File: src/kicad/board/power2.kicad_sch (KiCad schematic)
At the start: 12 parts, among them Q1 DMG2301L, SW6 Enable BAT, U3 BQ25172

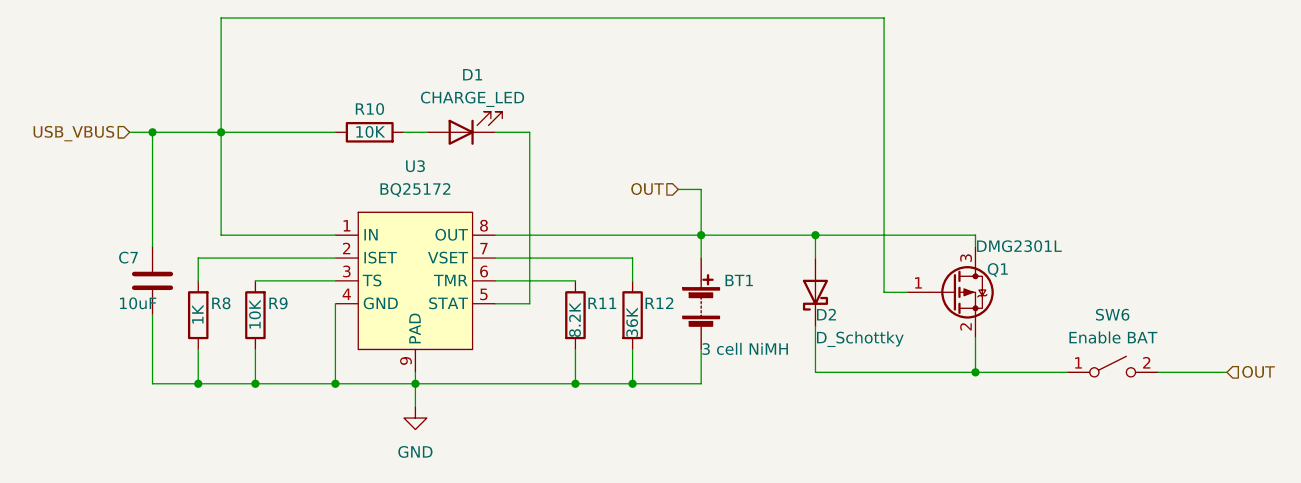
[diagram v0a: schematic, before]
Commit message: update wip
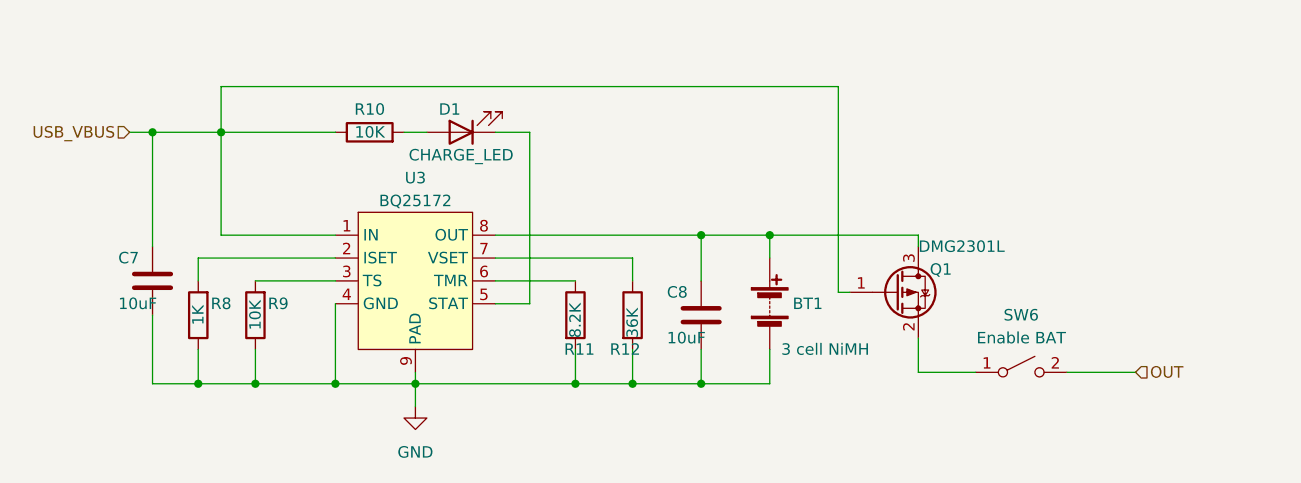
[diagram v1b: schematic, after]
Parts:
- removed D2: D_Schottky, symbol Device:D_Schottky
- added C8: 10uF, Capacitor_SMD:C_0805_2012Metric, symbol Device:C
- D1: footprint (none) -> LED_SMD:LED_0805_2012Metric
- U3: footprint (none) -> Library:BQ25172
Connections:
- net GND: now also C8.2
- net OUT: no longer BT1.1 (+), Q1.3 (D), U3.8 (OUT)
- new net: BT1.1 (+), C8.1, Q1.3 (D), U3.8 (OUT)
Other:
- moved on the sheet: BT1, Q1, SW6
